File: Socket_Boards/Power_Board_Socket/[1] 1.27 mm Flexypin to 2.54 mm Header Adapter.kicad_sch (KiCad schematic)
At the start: 2 parts

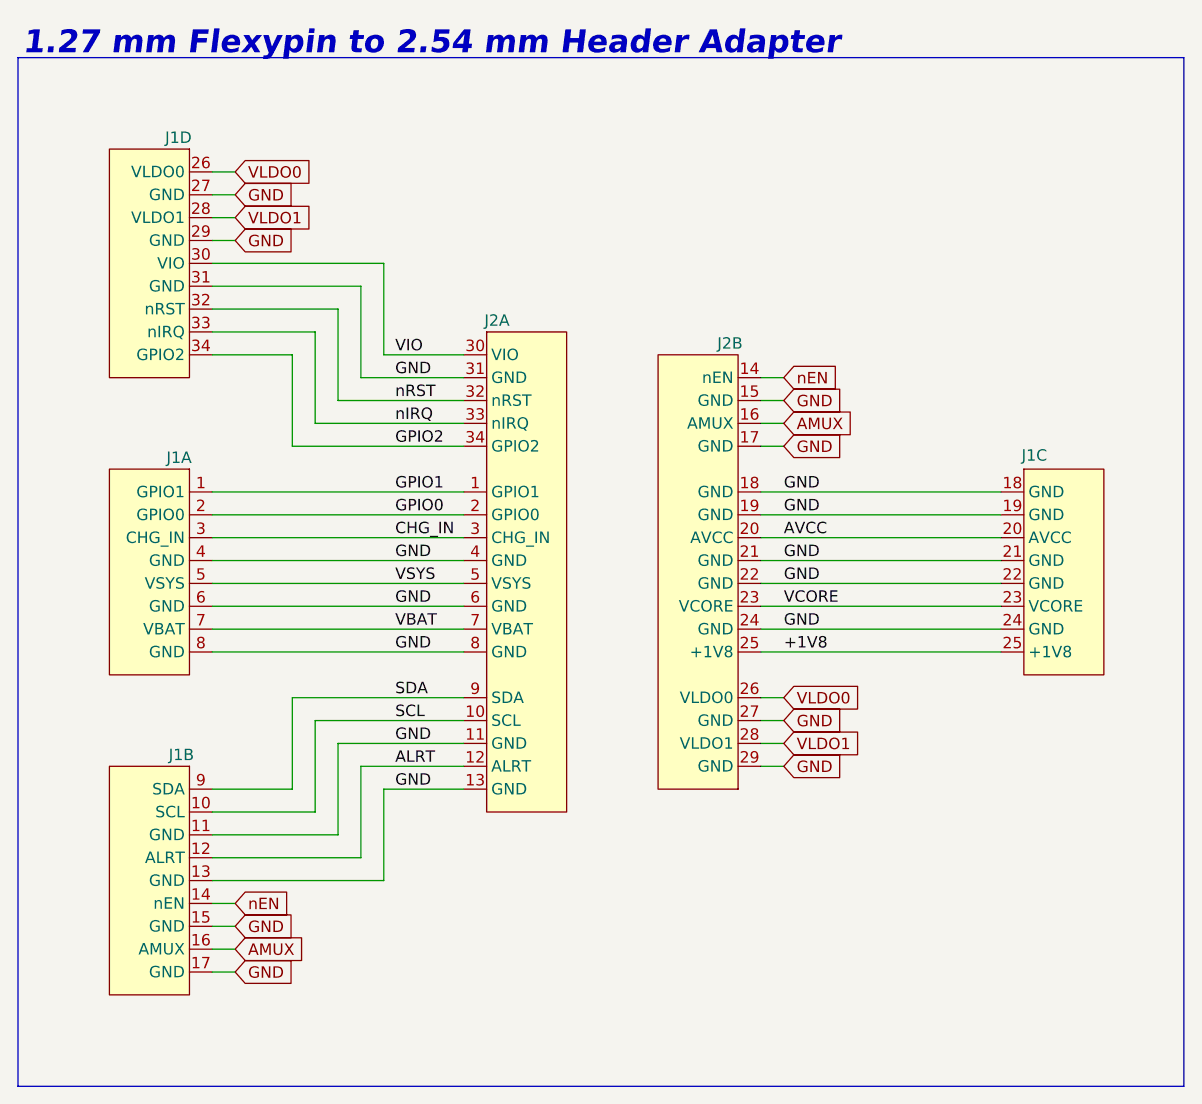
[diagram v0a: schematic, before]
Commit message: Big push. Fixed the issues that were pending. See github
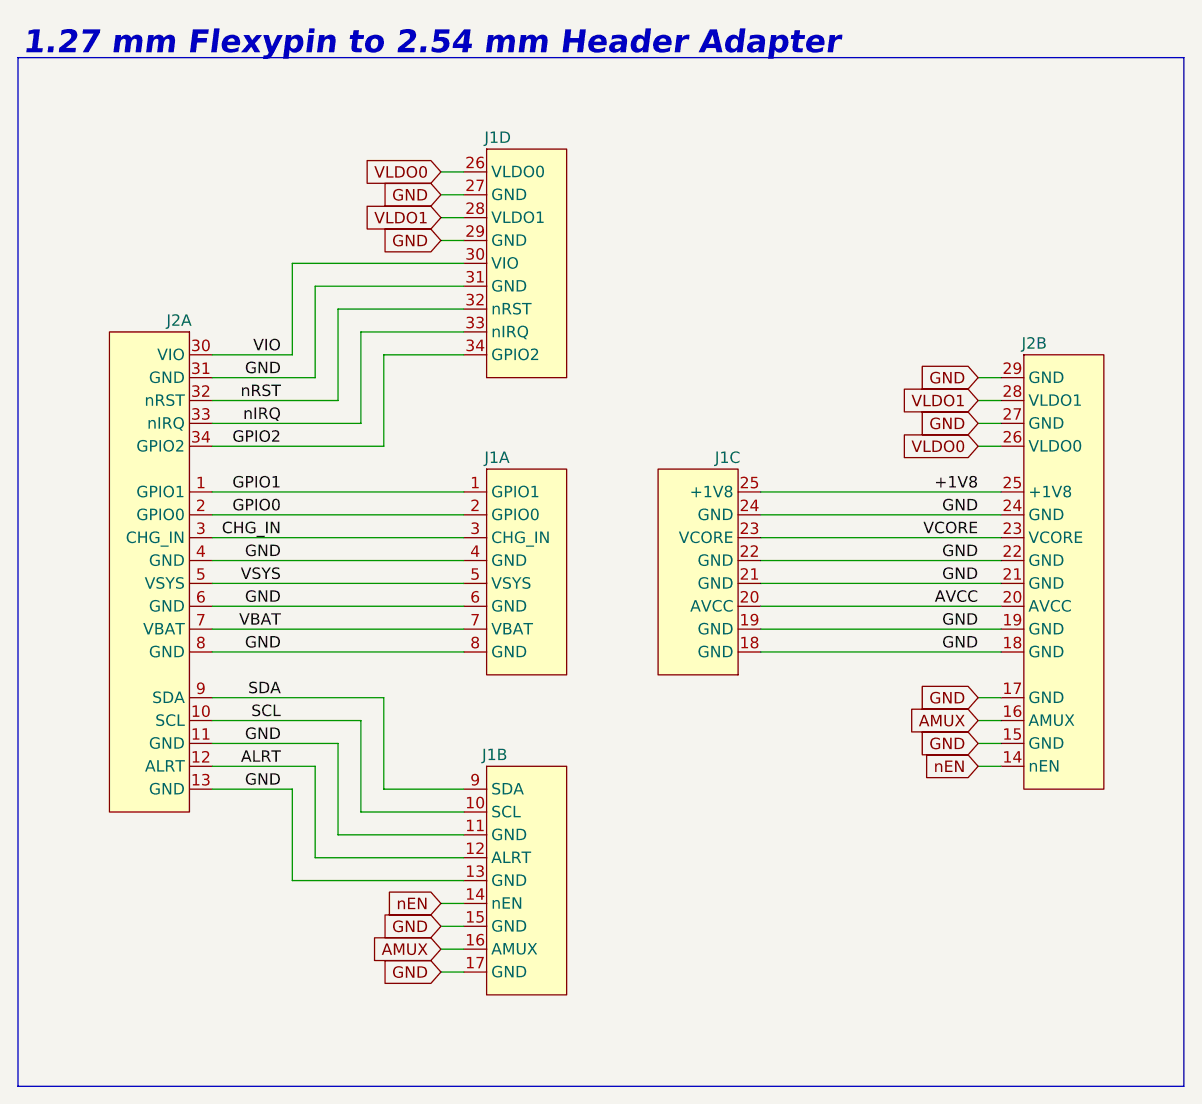
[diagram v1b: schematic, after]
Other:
- moved on the sheet: J1A, J1B, J1C, J1D, J2A, J2B

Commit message: Final revision and production files
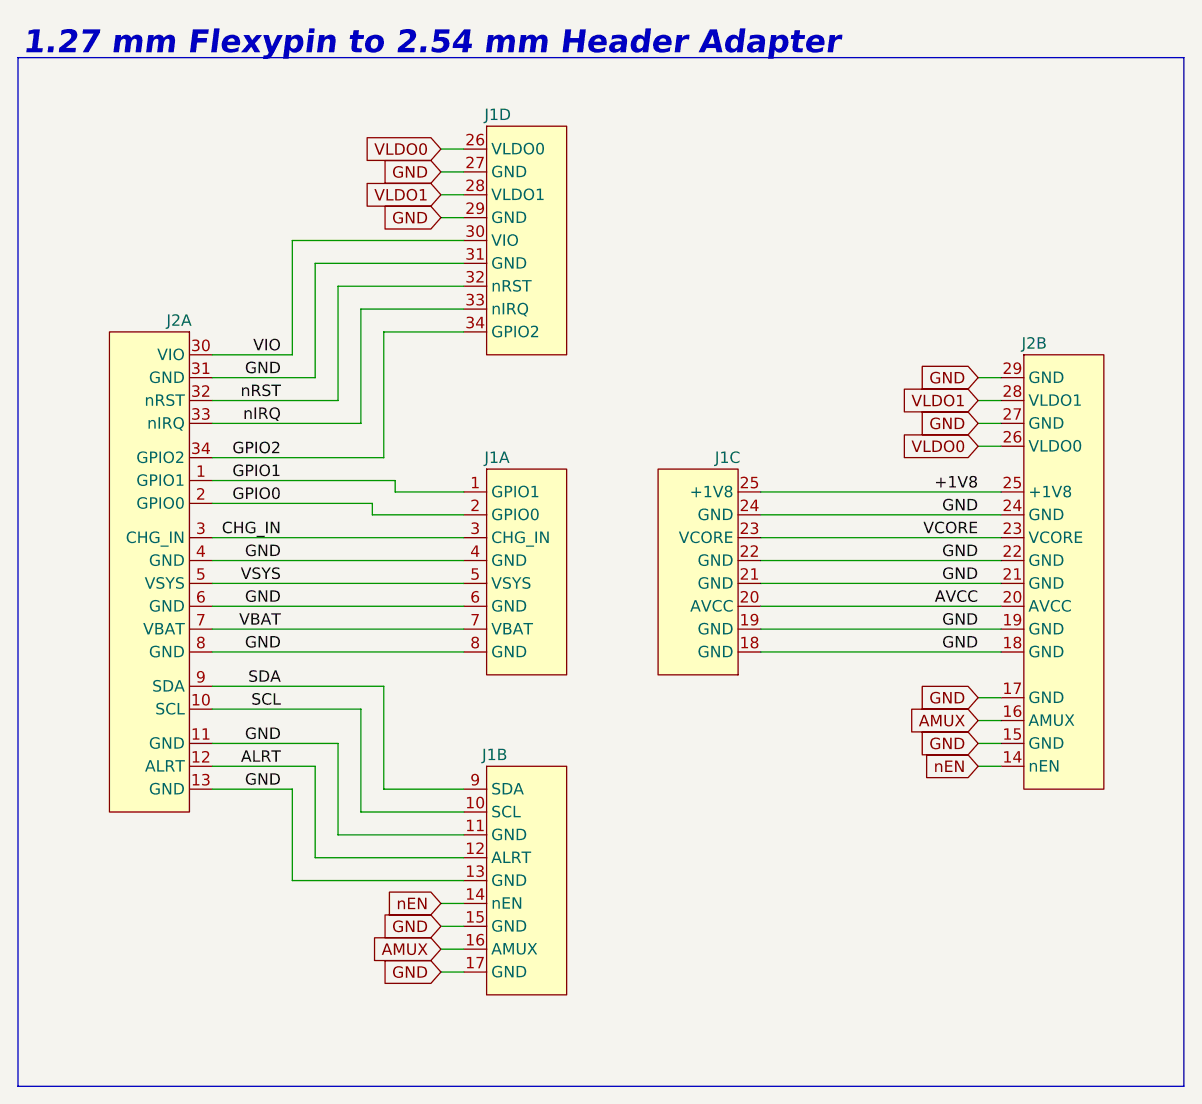
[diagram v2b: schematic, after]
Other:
- moved on the sheet: J1D
